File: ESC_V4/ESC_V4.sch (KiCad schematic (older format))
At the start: 45 parts, among them J1 Motor Power, J2 12V Power, J3 Motor Inputs, J4 Sensor Outputs, J5 Phase A, J6 Phase B, J7 Phase C, Q1 MOSFET NPN, Q2 MOSFET NPN, Q3 MOSFET NPN, Q4 MOSFET NPN, Q5 MOSFET NPN, Q6 MOSFET NPN, U1 TLV7044PWR, U2 LF2136BTR

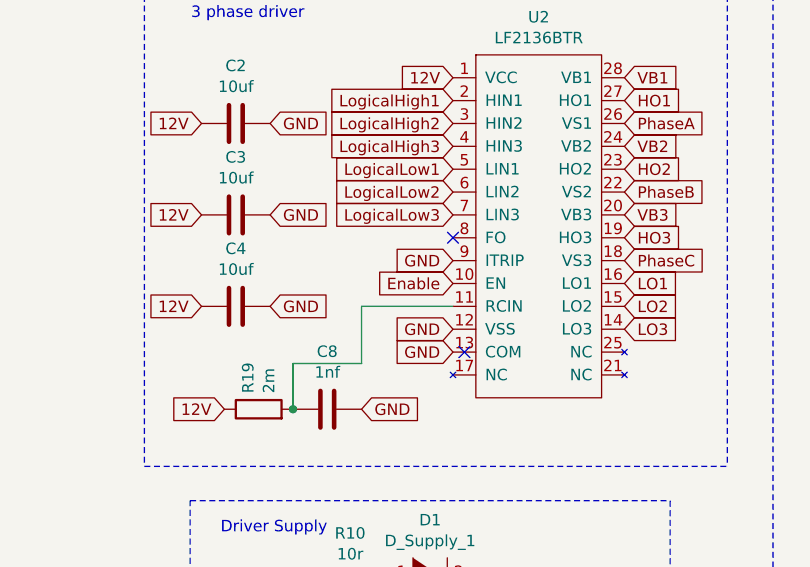
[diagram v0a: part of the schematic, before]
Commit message: Potentially finished layout
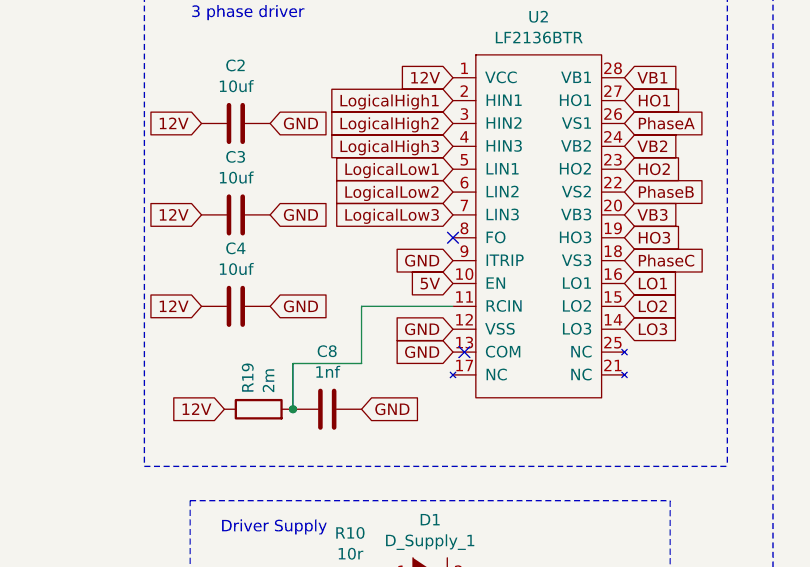
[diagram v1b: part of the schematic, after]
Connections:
- net Enable is gone; now on net 5V: U2.10 (EN)
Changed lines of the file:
@@
 AnalogComparator
 Text GLabel 6650 2600 0    50   Input ~ 0
-Enable
+5V
 $Comp
 L Connector:Conn_01x06_Female J3
